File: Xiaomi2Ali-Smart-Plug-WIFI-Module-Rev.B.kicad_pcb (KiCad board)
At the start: 2 copper layers, 34.8 x 47 mm, 18 parts, among them J1 Conn_01x07, J2 Conn_01x03, SW1 SW_Push

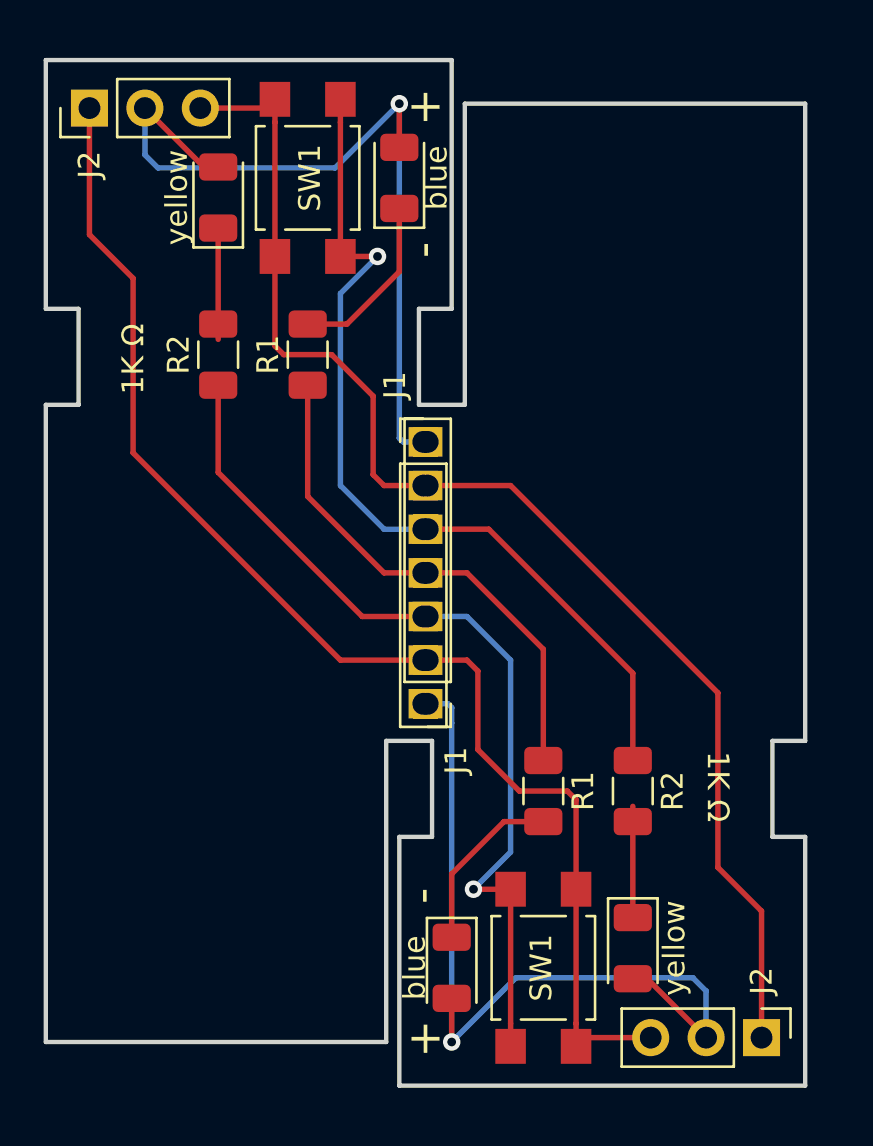
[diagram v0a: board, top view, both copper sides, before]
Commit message: Updated: 2019-02-20 16:21:37
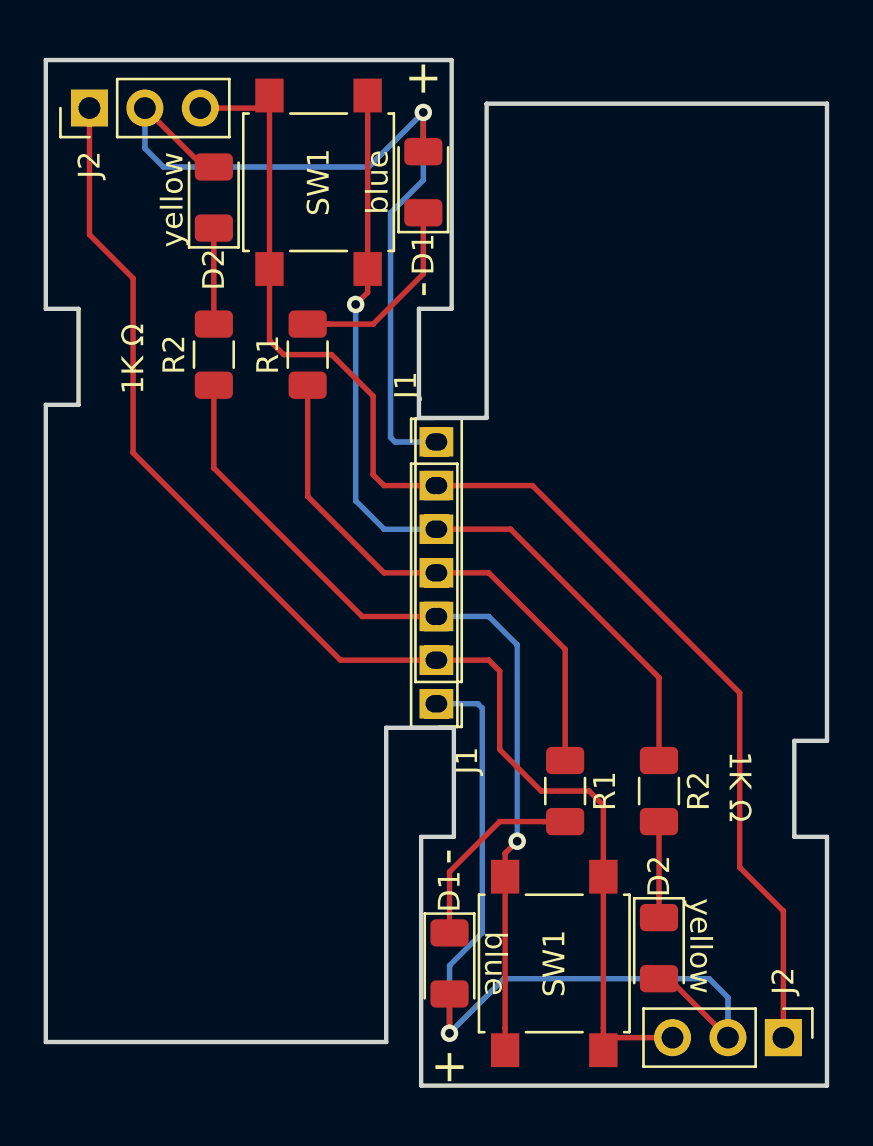
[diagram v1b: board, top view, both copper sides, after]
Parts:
- removed the J1 at (143.3, 87.5)
- removed the J1 at (143.5, 99.5)
- removed the SW1 at (148.8, 111.6)
- removed the SW1 at (138.0, 75.4)
- removed blue: LED_blue, LED_SMD:LED_1206_3216Metric
- removed yellow: LED_yellow, LED_SMD:LED_1206_3216Metric
- added D1: LED_blue, LED_SMD:LED_1206_3216Metric, F.Cu at (144.5, 111.4)
- added D2: LED_yellow, LED_SMD:LED_1206_3216Metric, F.Cu at (154.1, 110.7)
- added J1: Conn_01x07, Connector_PinHeader_2.00mm:PinHeader_1x07_P2.00mm_Vertical, F.Cu at (144.0, 99.5)
- added J1: Conn_01x07, Connector_PinHeader_2.00mm:PinHeader_1x07_P2.00mm_Vertical, F.Cu at (143.8, 87.5)
- added SW1: SW_Push, Button_Switch_SMD:SW_SPST_B3S-1000, F.Cu at (149.3, 111.4)
- added SW1: SW_Push, Button_Switch_SMD:SW_SPST_B3S-1000, F.Cu at (138.5, 75.6)
- moved R2 1.20 mm to (154.1, 103.5)
- moved D1 1.12 mm to (143.3, 75.6)
- moved J2 1.00 mm to (159.8, 114.8)
- moved R1 1.00 mm to (149.8, 103.5)
- moved REF** 1.00 mm to (153.8, 86.2)
- moved REF** 1.00 mm to (153.8, 77.0)
- moved D2 0.20 mm to (133.7, 76.3)
- moved R2 0.20 mm to (133.7, 83.5)
- renumbered blue to D1, yellow to D2
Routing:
- net Net-(J1-Pad3): track 24.9 -> 22.5 mm
- net VCC: track 38.2 -> 39.4 mm
- net Net-(D1-Pad1): track 8.09 -> 9.05 mm
- net (no net): track 163.9 -> 164.8 mm
- net GND: track 26.4 -> 27.2 mm
- net Net-(D2-Pad1): track 5.10 -> 4.40 mm
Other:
- board size 34.8 x 47 mm -> 35.8 x 47 mm
- board text added: "blue"
- board text added: "yellow"
